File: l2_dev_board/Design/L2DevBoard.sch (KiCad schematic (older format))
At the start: 20 parts, among them P101 CONN_10X2, P102 CONN_10X2, P103 CONN_10X2, P104 CONN_10X2, P105 CONN_10X2, P106 CONN_10X2, P107 CONN_10X2, P108 CONN_10X2, P109 CONN_10X2, P110 CONN_10X2, P111 CONN_10X2, P112 CONN_10X2, P113 CONN_10X2, P114 CONN_10X2, P115 CONN_10X2, U101 ASE_20MHZ

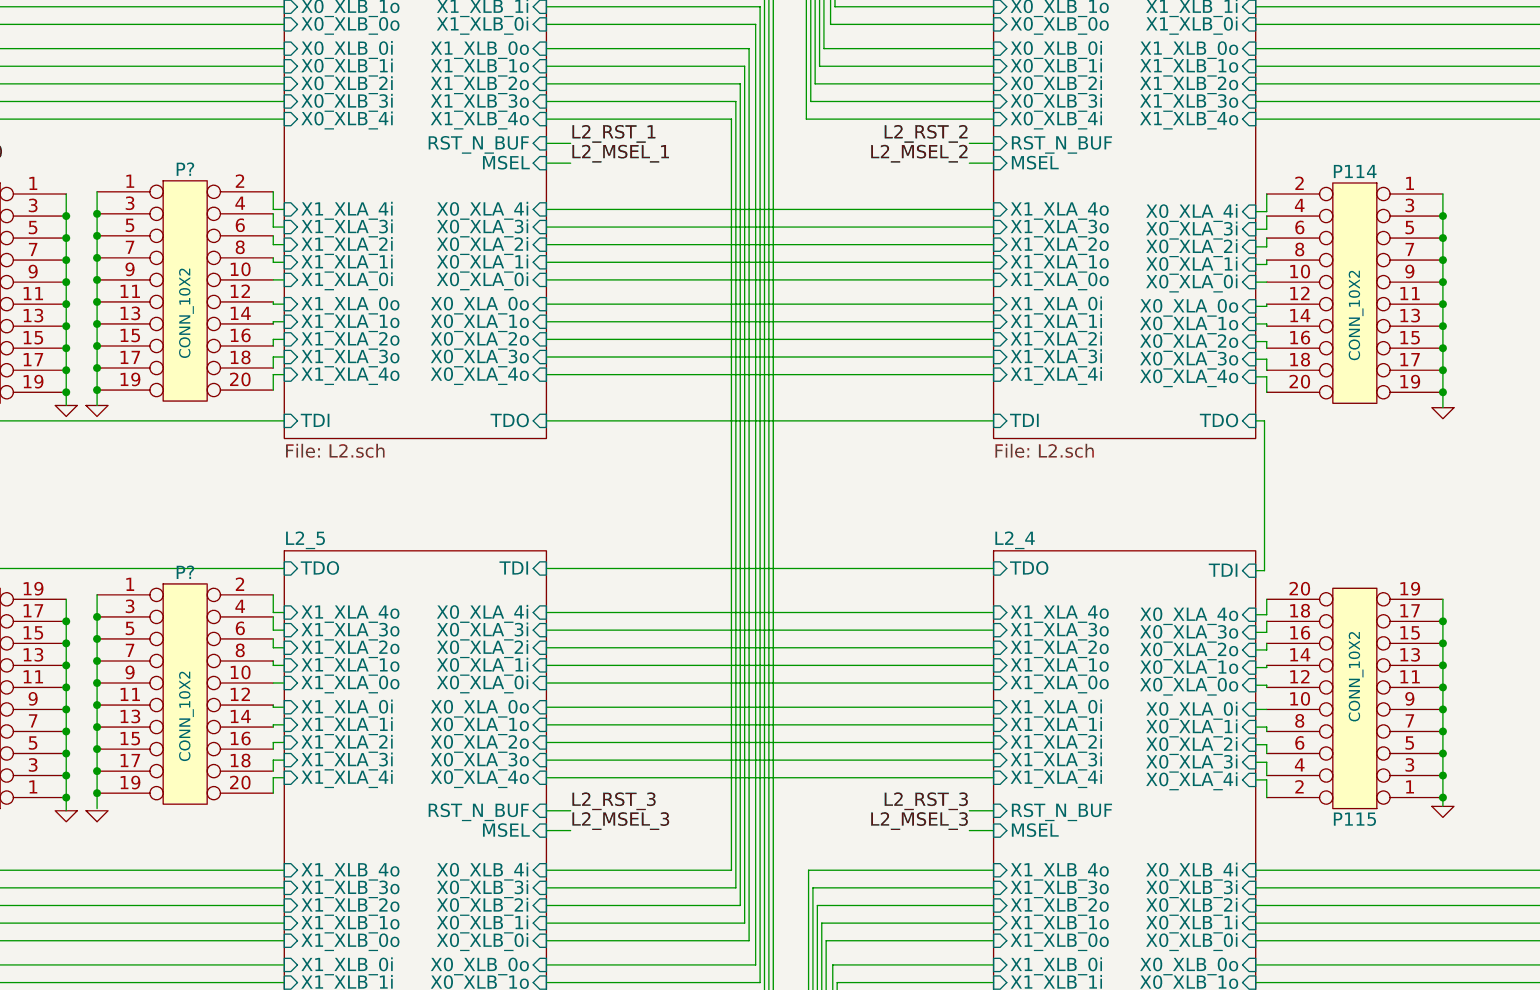
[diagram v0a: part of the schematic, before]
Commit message: new design with heirachial and new libraries
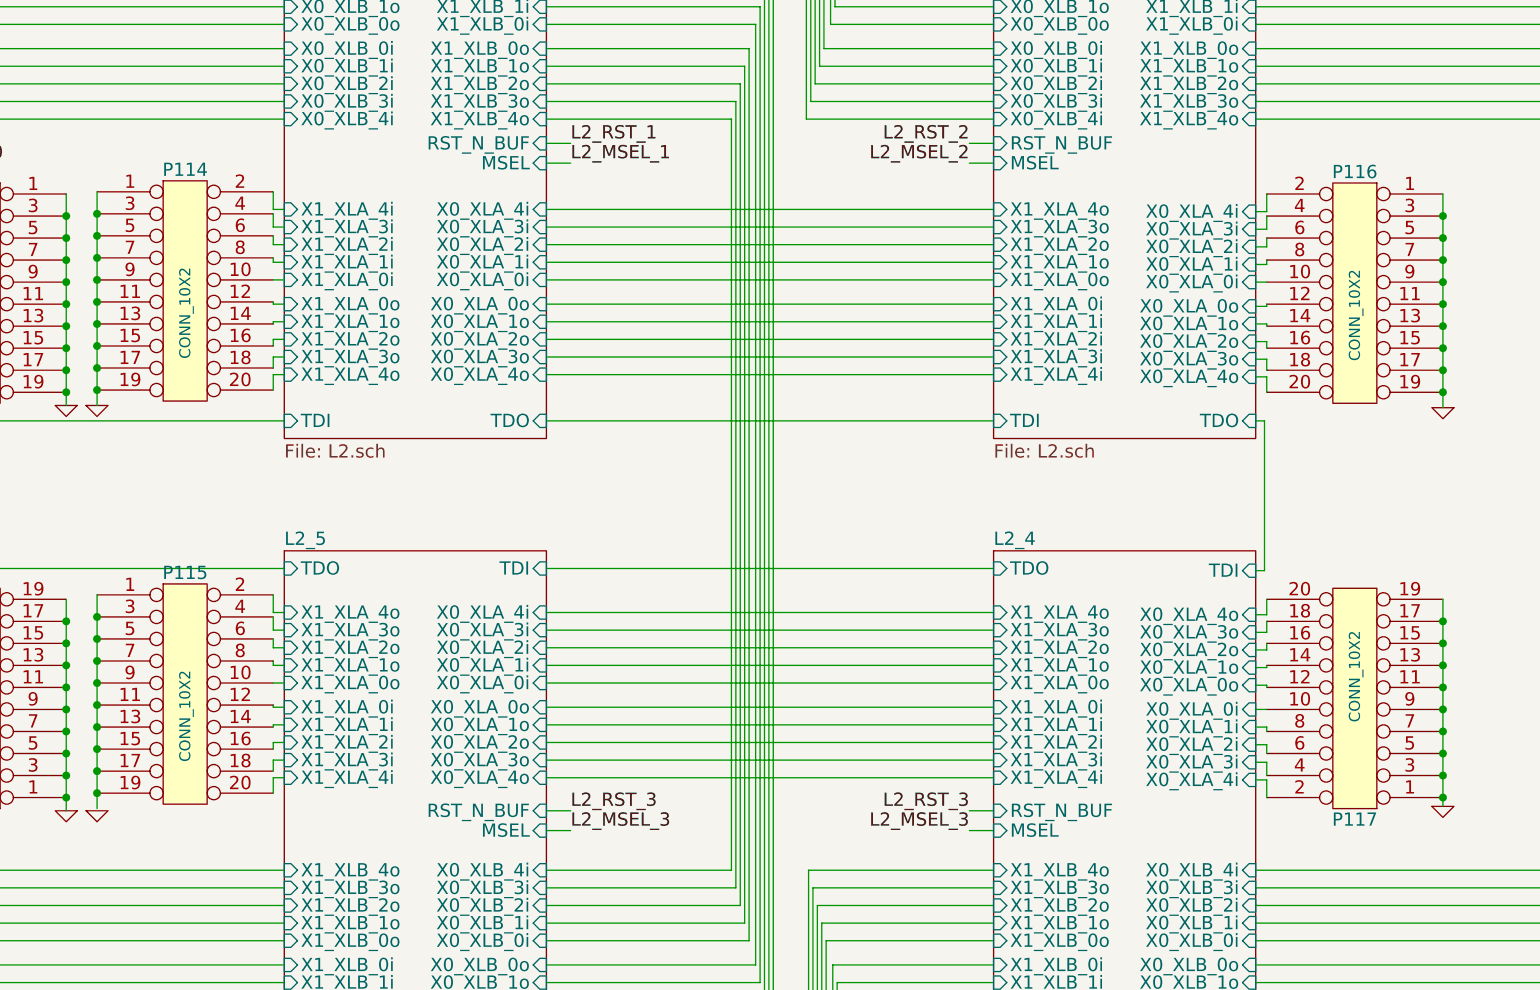
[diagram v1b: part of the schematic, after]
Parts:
- gave numbers to parts that had none: 2
- renumbered P114 to P116, P115 to P117
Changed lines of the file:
@@
-EESchema Schematic File Version 2  date 29/07/2011 09:19:43
+EESchema Schematic File Version 2  date 29/07/2011 14:29:23
 LIBS:power
 LIBS:device
@@
 Connection ~ 9160 5710
 $Comp
-L CONN_10X2 P?
+L CONN_10X2 P115
 U 1 1 4E326CFB
 P 9560 5260
-F 0 "P?" H 9560 5810 60  0000 C CNN
+F 0 "P115" H 9560 5810 60  0000 C CNN
 F 1 "CONN_10X2" V 9560 5160 50  0000 C CNN
 	1    9560 5260
@@
 $EndComp
 $Comp
-L GND #PWR?
+L GND #PWR01
 U 1 1 4E326CFA
 P 9160 5790
-F 0 "#PWR?" H 9160 5790 30  0001 C CNN
+F 0 "#PWR01" H 9160 5790 30  0001 C CNN
 F 1 "GND" H 9160 5720 30  0001 C CNN
 	1    9160 5790
@@
 $EndComp
 $Comp
-L GND #PWR?
+L GND #PWR02
 U 1 1 4E318DA5
 P 9160 3950
-F 0 "#PWR?" H 9160 3950 30  0001 C CNN
+F 0 "#PWR02" H 9160 3950 30  0001 C CNN
 F 1 "GND" H 9160 3880 30  0001 C CNN
 	1    9160 3950
@@
 $EndComp
 $Comp
-L CONN_10X2 P?
+L CONN_10X2 P114
 U 1 1 4E318DA4
 P 9560 3430
-F 0 "P?" H 9560 3980 60  0000 C CNN
+F 0 "P114" H 9560 3980 60  0000 C CNN
 F 1 "CONN_10X2" V 9560 3330 50  0000 C CNN
 	1    9560 3430
@@
 L2_MSEL_0
 $Comp
-L GND #PWR01
+L GND #PWR03
 U 1 1 4E31602E
 P 8000 9540
-F 0 "#PWR01" H 8000 9540 30  0001 C CNN
+F 0 "#PWR03" H 8000 9540 30  0001 C CNN
 F 1 "GND" H 8000 9470 30  0001 C CNN
 	1    8000 9540
@@
 $EndComp
 $Comp
-L GND #PWR02
+L GND #PWR04
 U 1 1 4E31602B
 P 8000 10610
-F 0 "#PWR02" H 8000 10610 30  0001 C CNN
+F 0 "#PWR04" H 8000 10610 30  0001 C CNN
 F 1 "GND" H 8000 10540 30  0001 C CNN
 	1    8000 10610
@@
 $EndComp
 $Comp
-L GND #PWR03
+L GND #PWR05
 U 1 1 4E316006
 P 4210 10610
-F 0 "#PWR03" H 4210 10610 30  0001 C CNN
+F 0 "#PWR05" H 4210 10610 30  0001 C CNN
 F 1 "GND" H 4210 10540 30  0001 C CNN
 	1    4210 10610
@@
 $EndComp
 $Comp
-L GND #PWR04
+L GND #PWR06
 U 1 1 4E315EE2
 P 4210 9540
-F 0 "#PWR04" H 4210 9540 30  0001 C CNN
+F 0 "#PWR06" H 4210 9540 30  0001 C CNN
 F 1 "GND" H 4210 9470 30  0001 C CNN
 	1    4210 9540
@@
 $EndSheet
 $Comp
-L CONN_10X2 P114
+L CONN_10X2 P116
 U 1 1 4E31377B
 P 14870 3440
-F 0 "P114" H 14870 3990 60  0000 C CNN
+F 0 "P116" H 14870 3990 60  0000 C CNN
 F 1 "CONN_10X2" V 14870 3340 50  0000 C CNN
 	1    14870 3440
@@
 $EndComp
 $Comp
-L GND #PWR05
+L GND #PWR07
 U 1 1 4E31377A
 P 15270 3960
-F 0 "#PWR05" H 15270 3960 30  0001 C CNN
+F 0 "#PWR07" H 15270 3960 30  0001 C CNN
 F 1 "GND" H 15270 3890 30  0001 C CNN
 	1    15270 3960
@@
 $EndComp
 $Comp
-L GND #PWR06
+L GND #PWR08
 U 1 1 4E313750
 P 15270 5770
-F 0 "#PWR06" H 15270 5770 30  0001 C CNN
+F 0 "#PWR08" H 15270 5770 30  0001 C CNN
 F 1 "GND" H 15270 5700 30  0001 C CNN
 	1    15270 5770
@@
 $EndComp
 $Comp
-L CONN_10X2 P115
+L CONN_10X2 P117
 U 1 1 4E31374F
 P 14870 5280
-F 0 "P115" H 14870 5830 60  0000 C CNN
+F 0 "P117" H 14870 5830 60  0000 C CNN
 F 1 "CONN_10X2" V 14870 5180 50  0000 C CNN
 	1    14870 5280
@@
 $EndComp
 $Comp
-L GND #PWR07
+L GND #PWR09
 U 1 1 4E3136DD
 P 5960 6960
-F 0 "#PWR07" H 5960 6960 30  0001 C CNN
+F 0 "#PWR09" H 5960 6960 30  0001 C CNN
 F 1 "GND" H 5960 6890 30  0001 C CNN
 	1    5960 6960
@@
 $EndComp
 $Comp
-L GND #PWR08
+L GND #PWR010
 U 1 1 4E313653
 P 5960 2790
-F 0 "#PWR08" H 5960 2790 30  0001 C CNN
+F 0 "#PWR010" H 5960 2790 30  0001 C CNN
 F 1 "GND" H 5960 2720 30  0001 C CNN
 	1    5960 2790
@@
 $EndComp
 $Comp
-L GND #PWR09
+L GND #PWR011
 U 1 1 4E31350D
 P 9020 3950
-F 0 "#PWR09" H 9020 3950 30  0001 C CNN
+F 0 "#PWR011" H 9020 3950 30  0001 C CNN
 F 1 "GND" H 9020 3880 30  0001 C CNN
 	1    9020 3950
@@
 $EndComp
 $Comp
-L GND #PWR010
+L GND #PWR012
 U 1 1 4E3134D9
 P 9020 5790
-F 0 "#PWR010" H 9020 5790 30  0001 C CNN
+F 0 "#PWR012" H 9020 5790 30  0001 C CNN
 F 1 "GND" H 9020 5720 30  0001 C CNN
 	1    9020 5790
@@
 $EndComp
 $Comp
-L GND #PWR011
+L GND #PWR013
 U 1 1 4E31341C
 P 2770 6970
-F 0 "#PWR011" H 2770 6970 30  0001 C CNN
+F 0 "#PWR013" H 2770 6970 30  0001 C CNN
 F 1 "GND" H 2770 6900 30  0001 C CNN
 	1    2770 6970
@@
 $EndComp
 $Comp
-L GND #PWR012
+L GND #PWR014
 U 1 1 4E3133EF
 P 2770 5780
-F 0 "#PWR012" H 2770 5780 30  0001 C CNN
+F 0 "#PWR014" H 2770 5780 30  0001 C CNN
 F 1 "GND" H 2770 5710 30  0001 C CNN
 	1    2770 5780
@@
 $EndComp
 $Comp
-L GND #PWR013
+L GND #PWR015
 U 1 1 4E31333A
 P 2770 3950
-F 0 "#PWR013" H 2770 3950 30  0001 C CNN
+F 0 "#PWR015" H 2770 3950 30  0001 C CNN
 F 1 "GND" H 2770 3880 30  0001 C CNN
 	1    2770 3950
@@
 $EndComp
 $Comp
-L GND #PWR014
+L GND #PWR016
 U 1 1 4E313320
 P 2770 2790
-F 0 "#PWR014" H 2770 2790 30  0001 C CNN
+F 0 "#PWR016" H 2770 2790 30  0001 C CNN
 F 1 "GND" H 2770 2720 30  0001 C CNN
 	1    2770 2790
@@
 $EndComp
 $Comp
-L GND #PWR015
+L GND #PWR017
 U 1 1 4E16FC64
 P 830 4120
-F 0 "#PWR015" H 830 4120 30  0001 C CNN
+F 0 "#PWR017" H 830 4120 30  0001 C CNN
 F 1 "GND" H 830 4050 30  0001 C CNN
 	1    830  4120
@@
 CLK_20M
 $Comp
-L GND #PWR016
+L GND #PWR018
 U 1 1 4E16F933
 P 1450 4080
-F 0 "#PWR016" H 1450 4080 30  0001 C CNN
+F 0 "#PWR018" H 1450 4080 30  0001 C CNN
 F 1 "GND" H 1450 4010 30  0001 C CNN
 	1    1450 4080
@@
 TDI
 $Comp
-L GND #PWR017
+L GND #PWR019
 U 1 1 4E159D56
 P 2100 2450
-F 0 "#PWR017" H 2100 2450 30  0001 C CNN
+F 0 "#PWR019" H 2100 2450 30  0001 C CNN
 F 1 "GND" H 2100 2380 30  0001 C CNN
 	1    2100 2450
